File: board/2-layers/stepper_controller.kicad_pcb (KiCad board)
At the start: 2 copper layers, 99 x 37 mm, 5 parts, among them U101 DRV8825, U102 DRV8825, U103 DRV8825, U201 STM32F103RG_LQFP64, U401 XC3S200A

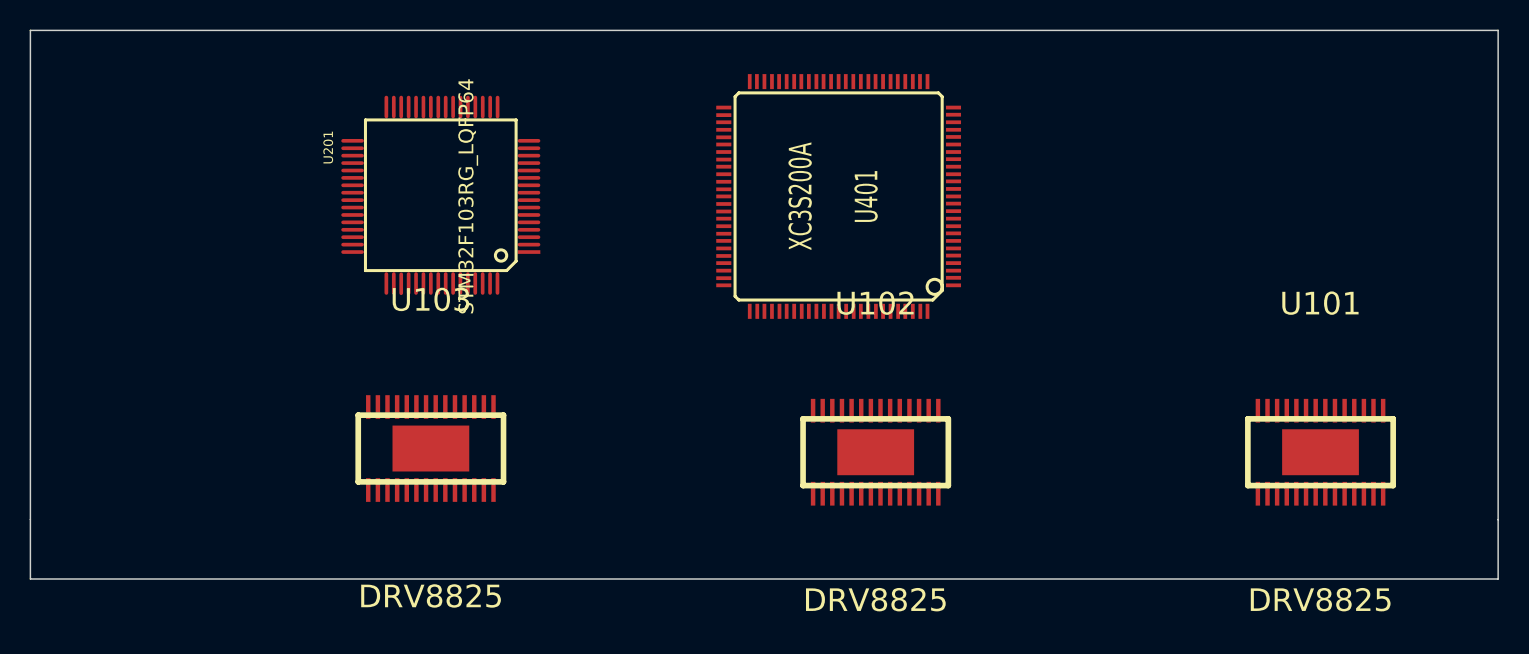
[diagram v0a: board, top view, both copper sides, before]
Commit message: added dac start routing
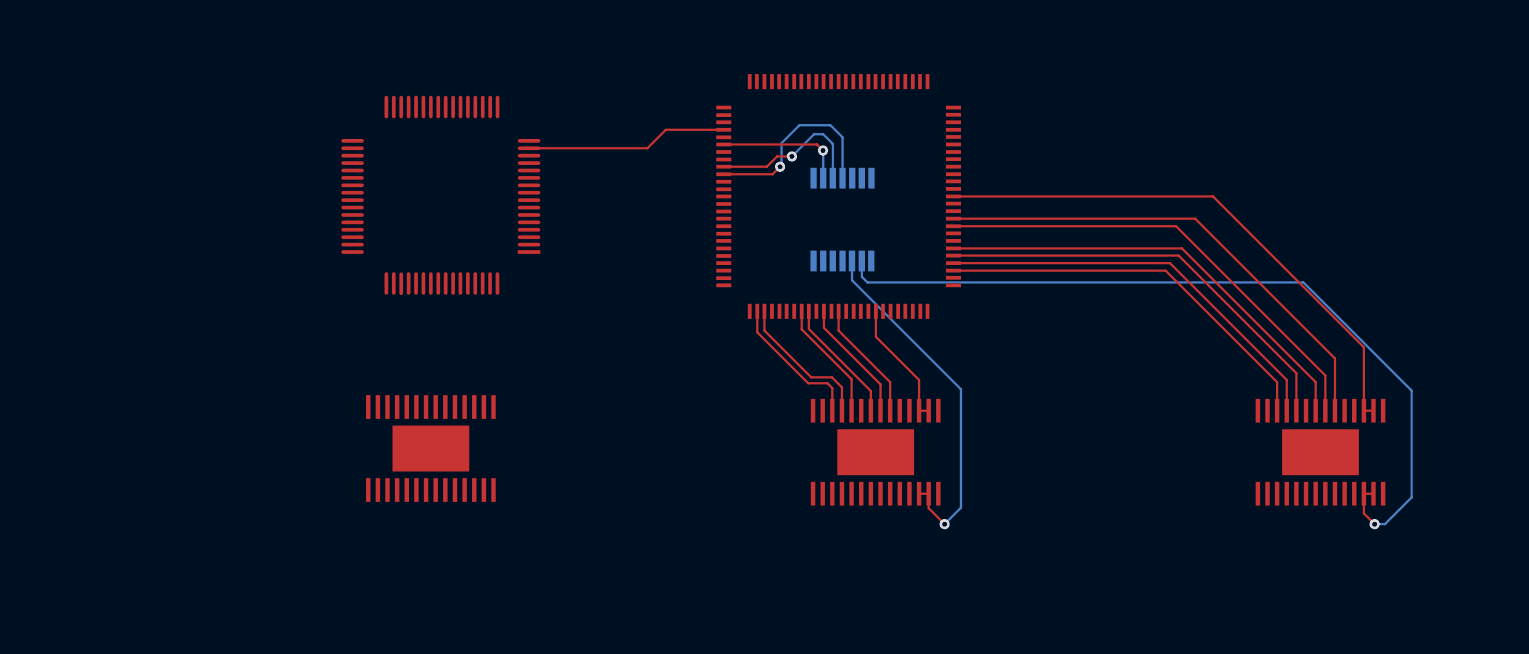
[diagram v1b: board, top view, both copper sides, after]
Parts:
- added U104: MAX5713/4/5-TSSOP14, SSOP14, B.Cu at (160.0, 99.1)
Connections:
- U101 pad 16: nRESET -> /FPGA/M2_RESET
- U101 pad 17: nRESET -> /FPGA/M2_RESET
- U101 pad 20: (no net) -> /FPGA/M2_DIR
- U101 pad 21: (no net) -> /FPGA/M2_EN
- U101 pad 22: STEP -> /FPGA/M2_STEP
- U101 pad 24: MODE0 -> /FPGA/M2_MODE0
- U101 pad 25: MODE1 -> /FPGA/M2_MODE1
- U101 pad 26: MODE2 -> /FPGA/M2_MODE2
- U102 pad 16: nRESET -> /FPGA/M1_RESET
- U102 pad 17: nRESET -> /FPGA/M1_RESET
- U102 pad 20: (no net) -> /FPGA/M1_DIR
- U102 pad 21: (no net) -> /FPGA/M1_EN
- U102 pad 22: STEP -> /FPGA/M1_STEP
- U102 pad 24: MODE0 -> /FPGA/M1_MODE0
- U102 pad 25: MODE1 -> /FPGA/M1_MODE1
- U102 pad 26: MODE2 -> /FPGA/M1_MODE2
- U201 pad 2: (no net) -> /STM32//CLR_DAC
- U401 pad 10: (no net) -> /FPGA/M2_DIR
- U401 pad 11: (no net) -> +3.3V
- U401 pad 13: (no net) -> /FPGA/M2_RESET
- U401 pad 3: (no net) -> /FPGA/M2_MODE2
- U401 pad 4: (no net) -> /FPGA/M2_MODE1
- U401 pad 5: (no net) -> /FPGA/M2_MODE0
- U401 pad 6: (no net) -> /FPGA/M2_STEP
- U401 pad 77: (no net) -> /FPGA/M1_MODE2
- U401 pad 78: (no net) -> /FPGA/M1_MODE1
- U401 pad 83: (no net) -> /FPGA/M1_MODE0
- U401 pad 84: (no net) -> /FPGA/M1_STEP
- U401 pad 86: (no net) -> /FPGA/M1_EN
- U401 pad 88: (no net) -> /FPGA/M1_DIR
- U401 pad 9: (no net) -> /FPGA/M2_EN
- U401 pad 93: (no net) -> /FPGA/M1_RESET
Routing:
- net /VRF_2: track 0.00 -> 54.8 mm, vias 0 -> 1
- net /FPGA/M2_RESET: track 0.00 -> 36.8 mm
- net /FPGA/M2_DIR: track 0.00 -> 33.2 mm
- net /FPGA/M2_EN: track 0.00 -> 31.6 mm
- net /FPGA/M2_STEP: track 0.00 -> 30.1 mm
- net /FPGA/M2_MODE0: track 0.00 -> 28.9 mm
- net /FPGA/M2_MODE1: track 0.00 -> 27.8 mm
- net /FPGA/M2_MODE2: track 0.00 -> 26.9 mm
- net /VRF_1: track 0.00 -> 24.4 mm, vias 0 -> 1
- net /FPGA/DONE: track 0.00 -> 13.6 mm
- net /FPGA/COM_CS: track 0.00 -> 13.3 mm, vias 0 -> 1
- net /FPGA/COM_CLK: track 0.00 -> 10.8 mm, vias 0 -> 1
- net /FPGA/M1_MODE1: track 0.00 -> 9.69 mm
- net /FPGA/M1_MODE2: track 0.00 -> 9.56 mm
- net /FPGA/COM_MOSI: track 0.00 -> 8.74 mm, vias 0 -> 1
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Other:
- board outline removed
